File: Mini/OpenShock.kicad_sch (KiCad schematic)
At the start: 40 parts, among them J1 USB_C_Receptacle_USB2.0, J2 Conn_01x03, J3 Conn_01x03, J4 Conn_01x06, J5 Conn_01x02, J6 Conn_01x04, SW1 KH-6X6X6H-TJ, SW2 KH-6X6X6H-TJ, SW3 KH-6X6X6H-TJ, U1 ESP32-S3-WROOM-1, U2 TPS7A2033PDBVR, U4 DL-TX1-433M

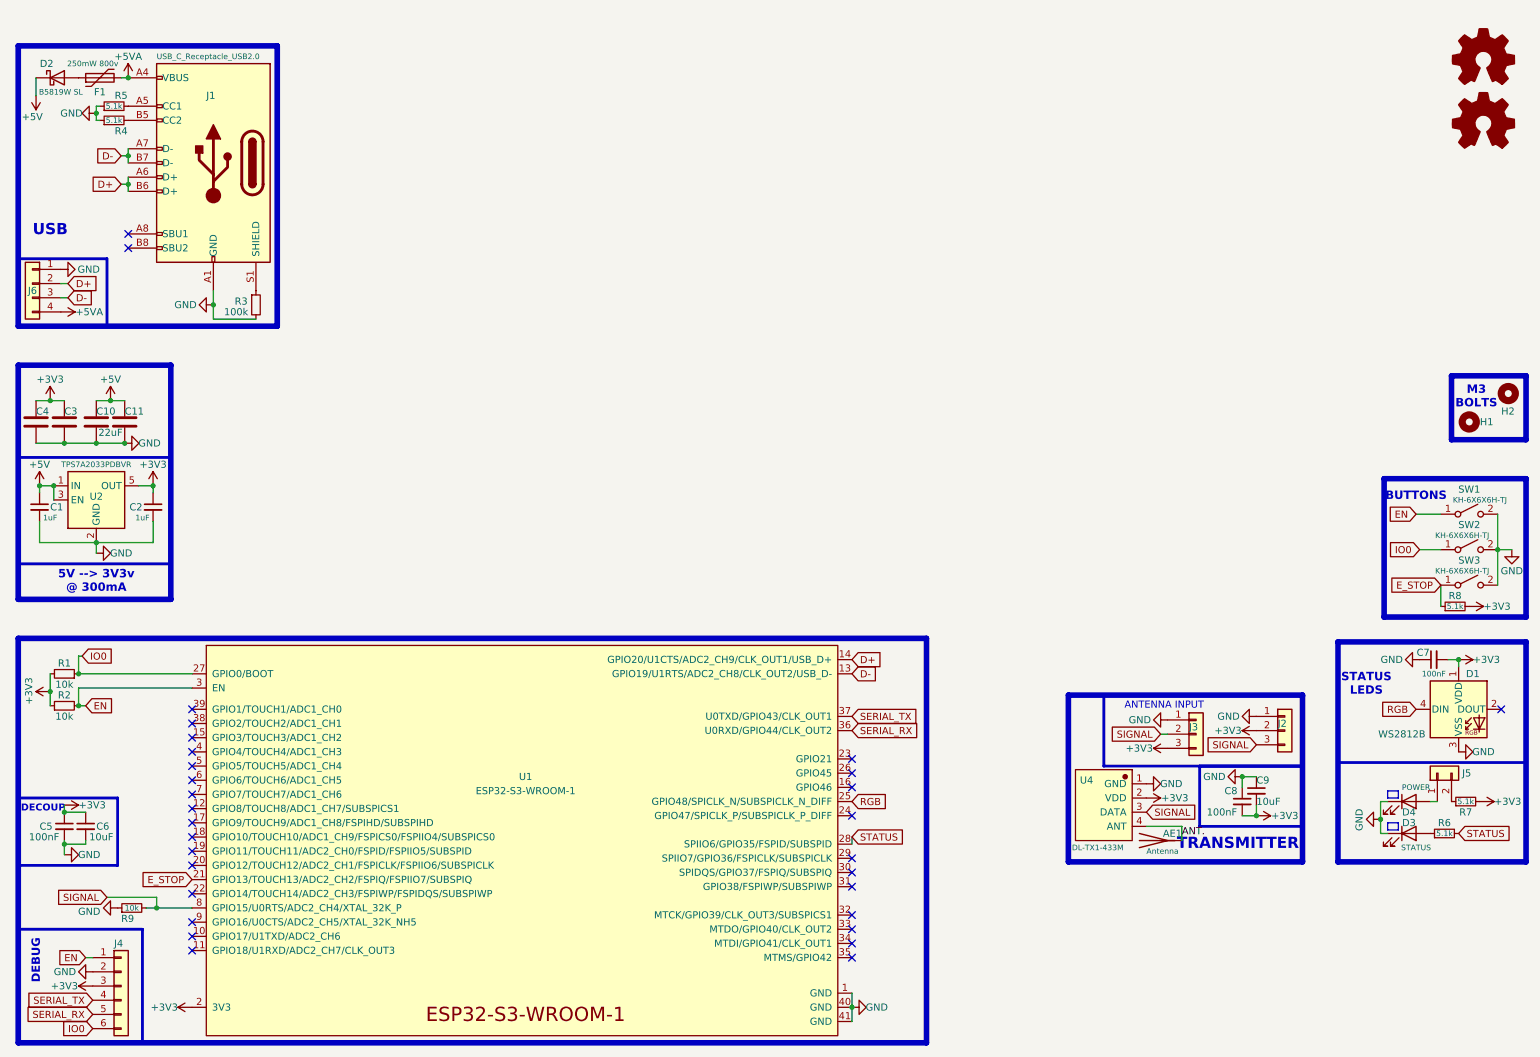
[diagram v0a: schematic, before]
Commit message: New Revision.
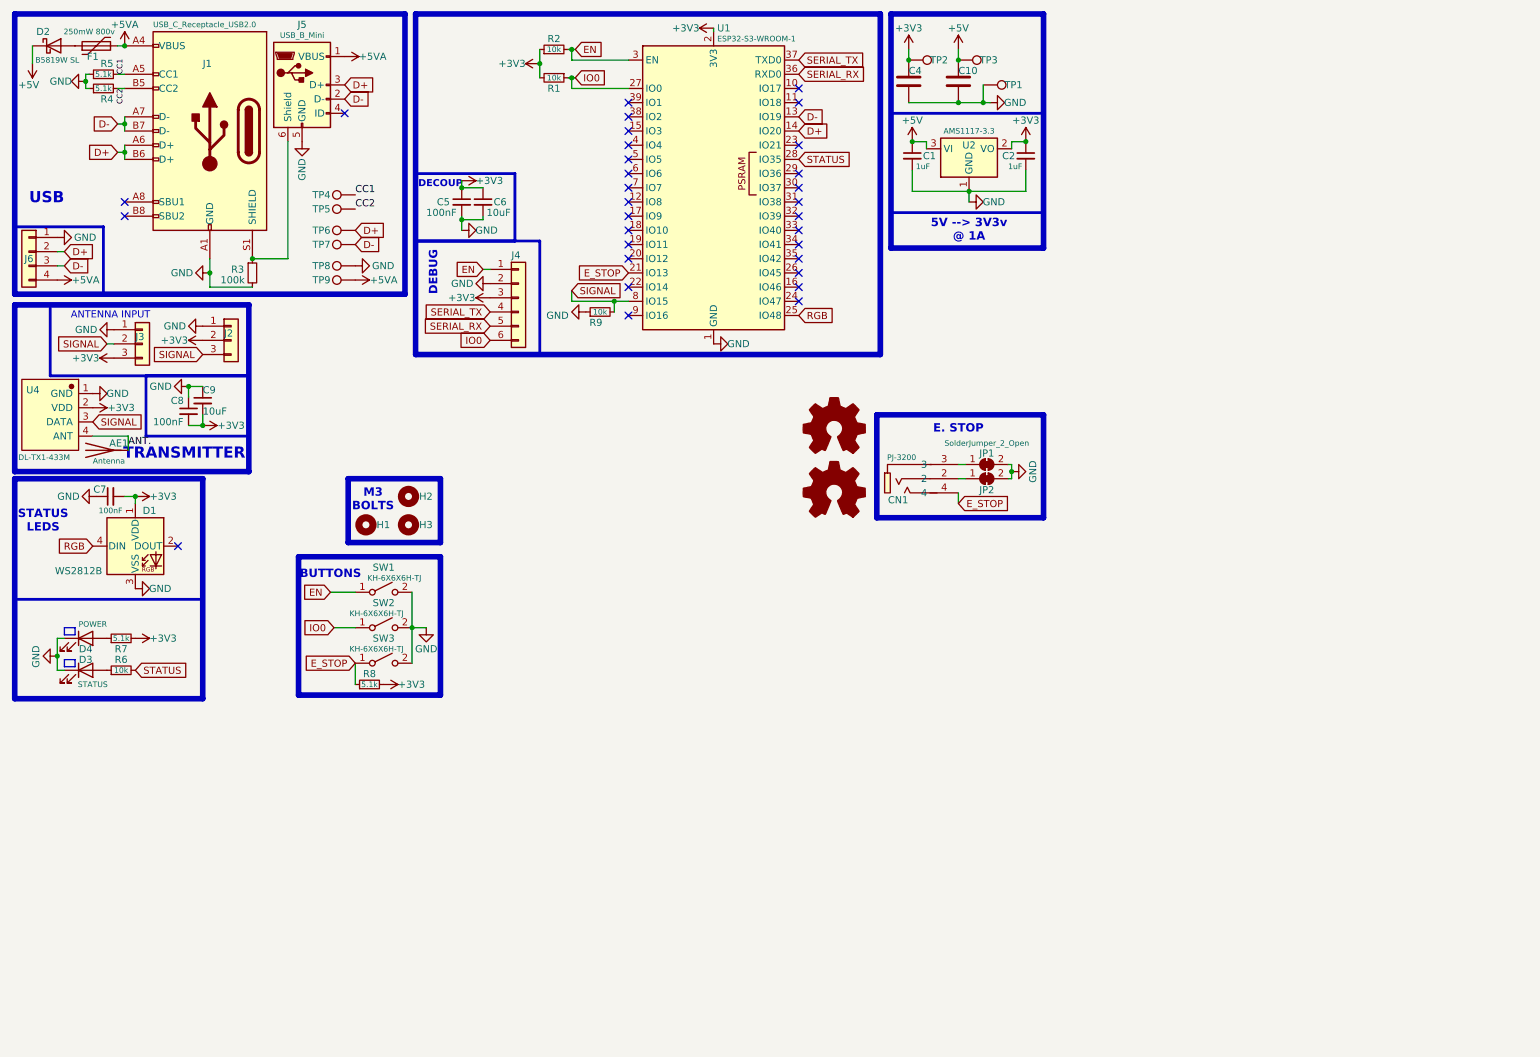
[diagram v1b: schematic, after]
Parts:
- removed C11, C3: 22uF, Capacitor_SMD:C_0603_1608Metric_Pad1.08x0.95mm_HandSolder, symbol Device:C
- removed J5: Conn_01x02, Connector_PinHeader_2.54mm:PinHeader_1x02_P2.54mm_Vertical, symbol Connector_Generic:Conn_01x02
- removed U1: ESP32-S3-WROOM-1, RF_Module:ESP32-S3-WROOM-1, symbol Espressif:ESP32-S3-WROOM-1
- removed U2: TPS7A2033PDBVR, PCM_Package_TO_SOT_SMD_AKL:SOT-23-5_HandSoldering, symbol Regulator_Linear:TPS7A0508PDBV
- added CN1: PJ-3200, EASYEDA Footprints:AUDIO-TH_PJ-3200, symbol EASYEDA Symbols:PJ-3200
- added H3: MountingHole, MountingHole:MountingHole_3.2mm_M3_ISO7380, symbol Mechanical:MountingHole
- added J5: USB_B_Mini, EASYEDA Footprints:MICRO-USB-TH_UX-150-ARG4, symbol Connector:USB_B_Mini
- added JP1, JP2: SolderJumper_2_Open, Jumper:SolderJumper-2_P1.3mm_Bridged_RoundedPad1.0x1.5mm, symbol Jumper:SolderJumper_2_Bridged
- added TP1, TP2, TP3, TP4, TP5, TP6, TP7, TP8, TP9: TestPoint, TestPoint:TestPoint_Pad_D1.5mm, symbol Connector:TestPoint
- added U1: ESP32-S3-WROOM-1, CustomFootprints:ESP32-S3-WROOM-1, symbol RF_Module:ESP32-S3-WROOM-1
- added U2: AMS1117-3.3, Package_TO_SOT_SMD:SOT-89-3_Handsoldering, symbol Regulator_Linear:AMS1117-3.3
- AE1: Alt. (none) -> https://aliexpress.com/item/1005005557947265.html
- C1, C2: footprint Capacitor_SMD:C_0603_1608Metric_Pad1.08x0.95mm_HandSolder -> Capacitor_SMD:C_0805_2012Metric_Pad1.18x1.45mm_HandSolder; LCSC C5189821 -> C215803
- C10, C4: footprint Capacitor_SMD:C_0603_1608Metric_Pad1.08x0.95mm_HandSolder -> Capacitor_SMD:C_0805_2012Metric_Pad1.18x1.45mm_HandSolder; LCSC C7432770 -> C98190
- C5, C7, C8: footprint Capacitor_SMD:C_0603_1608Metric_Pad1.08x0.95mm_HandSolder -> Capacitor_SMD:C_0805_2012Metric_Pad1.18x1.45mm_HandSolder; LCSC C6119861 -> C476766
- C6, C9: footprint Capacitor_SMD:C_0603_1608Metric_Pad1.08x0.95mm_HandSolder -> Capacitor_SMD:C_0805_2012Metric_Pad1.18x1.45mm_HandSolder; LCSC C380316 -> C1713
- R6: value 5.1k -> 10k
- U4: SuppliersPartNumber C381160 -> (none); uuid std:a9d6032d7d124c34850e850e6d051323 -> (none)
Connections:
- net +3V3: now also TP2.1, U1.2 (3V3), U2.2 (VO)
- net +5V: now also TP3.1, U2.3 (VI)
- net +5VA: now also J5.1 (VBUS), TP9.1
- net D+: now also J5.3 (D+), TP6.1, U1.14 (IO20)
- net D-: now also J5.2 (D-), TP7.1, U1.13 (IO19)
- net EN: now also U1.3 (EN)
- net E_STOP: now also CN1.4, U1.21 (IO13)
- net GND: now also J5.5 (GND), JP1.2 (B), JP2.2 (B), TP1.1, TP8.1, U1.1 (GND), U1.40 (GND), U1.41 (GND), U2.1 (GND)
- net IO0: now also U1.27 (IO0)
- net RGB: now also U1.25 (IO48)
- net SERIAL_RX: now also U1.36 (RXD0)
- net SERIAL_TX: now also U1.37 (TXD0)
- net SIGNAL: now also U1.8 (IO15)
- net STATUS: now also U1.28 (IO35)
- net at R7.1: now also D4.2 (A)
- net CC2: now reaches J1.B5 (CC2), R4.2
- net CC2: now also TP5.1
- net CC1: now reaches J1.A5 (CC1), R5.2
- net CC1: now also TP4.1
- net at J1.S1 (SHIELD), R3.1: now also J5.6 (Shield)
- new net: CN1.2, JP2.1 (A)
- new net: CN1.3, JP1.1 (A)
- no-connect marks 30 -> 31
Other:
- note added: "5V --> 3V3v @ 1A"
- note added: "E. STOP"
- note removed: "5V --> 3V3v @ 300mA"
- moved on the sheet: AE1, C1, C10, C2, C4, C5, C6, C7, C8, C9, D1, D2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
